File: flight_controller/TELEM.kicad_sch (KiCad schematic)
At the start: 18 parts, among them J13 A1257WV-S-6P-LCP, J14 A1257WV-S-6P-LCP, J15 A1257WV-S-6P-LCP

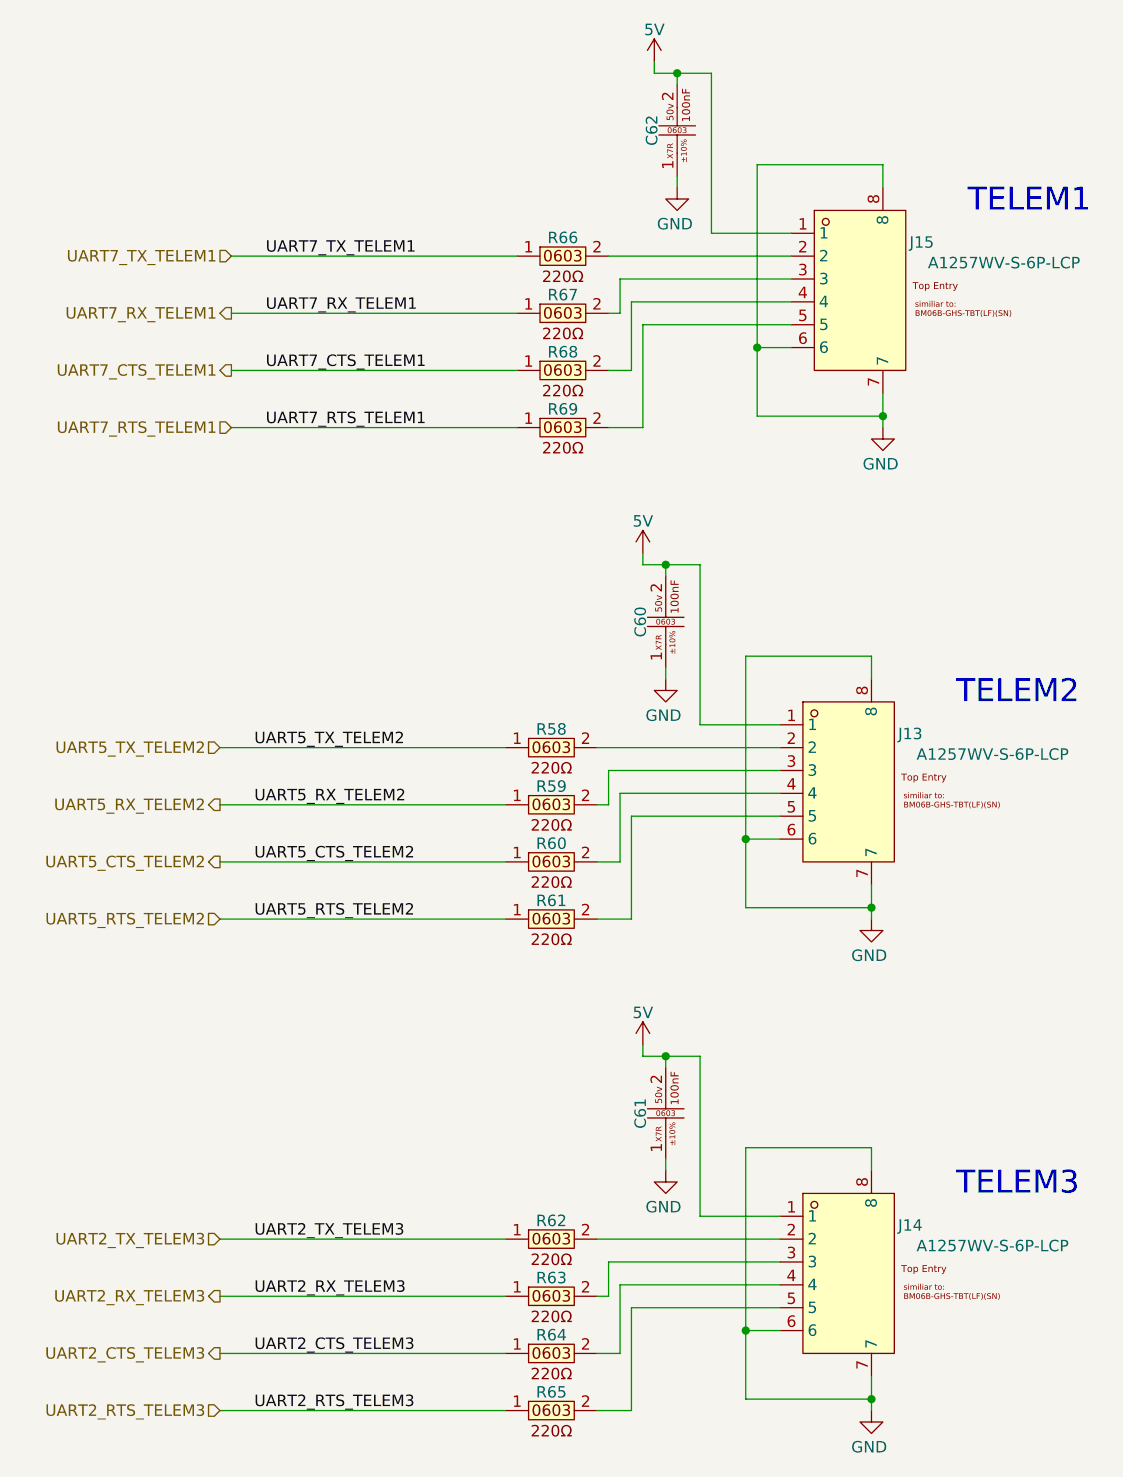
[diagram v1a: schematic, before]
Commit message: Revert to state of commit 2458262 moved all to components to top
Reverts commits: d012532, 3d9c600, 58bc0ac
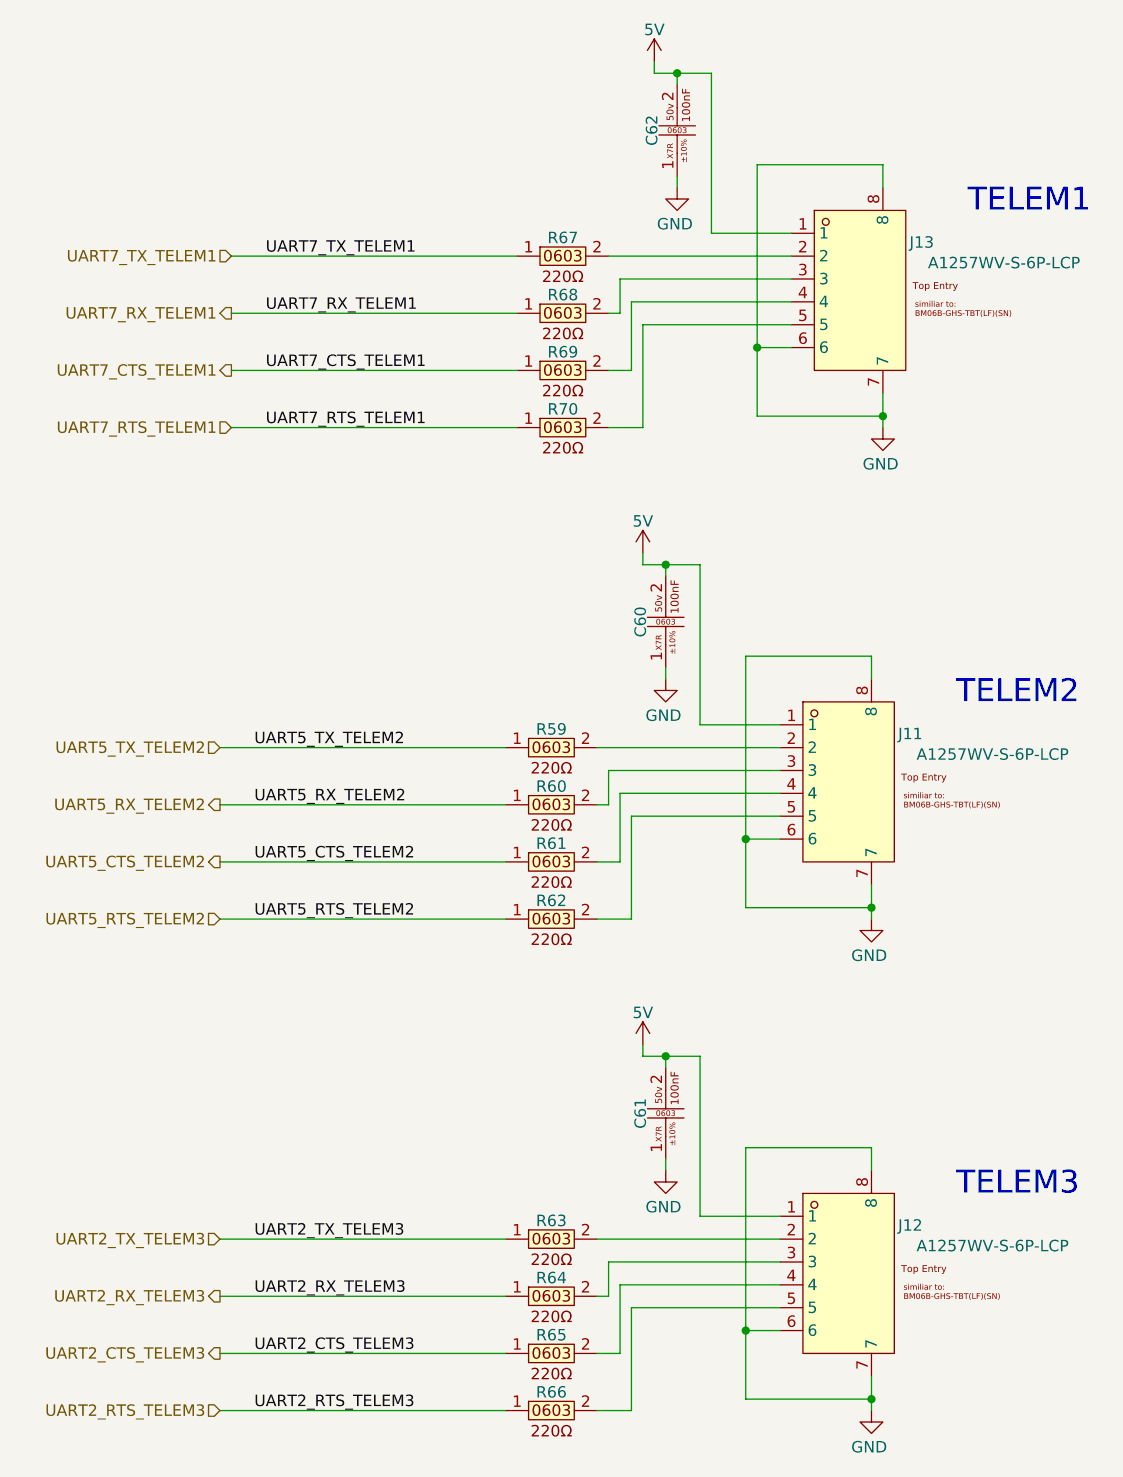
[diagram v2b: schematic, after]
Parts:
- renumbered J13 to J11, J14 to J12, J15 to J13, R58 to R59, R59 to R60, R60 to R61, R61 to R62, R62 to R63, R63 to R64, R64 to R65, R65 to R66, R66 to R67, R67 to R68, R68 to R69, R69 to R70
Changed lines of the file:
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@@
+		(polyline
+			(pts
+				(xy 68.58 129.54) (xy 68.58 181.61) (xy 148.59 181.61) (xy 148.59 129.54)
+			)
+			(stroke
+				(width 0)
+				(type dash)
+			)
+			(fill
+				(type none)
+			)
+		)
+	)
+	(rule_area
 		(polyline
 			(pts
@@
 			(pts
 				(xy 79.375 74.93) (xy 79.375 127) (xy 173.99 127.635) (xy 173.99 74.93)
-			)
-			(stroke
-				(width 0)
-				(type dash)
-			)
-			(fill
-				(type none)
-			)
-		)
-	)
-	(rule_area
-		(polyline
-			(pts
-				(xy 68.58 129.54) (xy 68.58 181.61) (xy 148.59 181.61) (xy 148.59 129.54)
 			)
 			(stroke
@@
 		(dnp no)
 		(fields_autoplaced yes)
-		(property "Reference" "R64"
+		(property "Reference" "R65"
 			(at 85.09 166.878 0)
 			(do_not_autoplace yes)
@@
 			(project "FP_BOARD"
 				(path "/17737359-1a8e-4237-8899-d9604030bc1d/ee742a7d-8184-434b-840f-4020f45cd711"
-					(reference "R64")
+					(reference "R65")
 					(unit 1)
 				)
@@
 		(on_board yes)
 		(dnp no)
-		(property "Reference" "#PWR0158"
+		(property "Reference" "#PWR0160"
 			(at 95.25 138.43 0)
 			(effects
@@
 			(project "FP_BOARD"
 				(path "/17737359-1a8e-4237-8899-d9604030bc1d/ee742a7d-8184-434b-840f-4020f45cd711"
-					(reference "#PWR0158")
+					(reference "#PWR0160")
 					(unit 1)
 				)
@@
 		(dnp no)
 		(fields_autoplaced yes)
-		(property "Reference" "R65"
+		(property "Reference" "R66"
 			(at 85.09 173.228 0)
 			(do_not_autoplace yes)
@@
 			(project "FP_BOARD"
 				(path "/17737359-1a8e-4237-8899-d9604030bc1d/ee742a7d-8184-434b-840f-4020f45cd711"
-					(reference "R65")
+					(reference "R66")
 					(unit 1)
 				)
@@
 		(dnp no)
 		(fields_autoplaced yes)
-		(property "Reference" "R60"
+		(property "Reference" "R61"
 			(at 85.09 112.268 0)
 			(do_not_autoplace yes)
@@
 			(project "FP_BOARD"
 				(path "/17737359-1a8e-4237-8899-d9604030bc1d/ee742a7d-8184-434b-840f-4020f45cd711"
-					(reference "R60")
+					(reference "R61")
 					(unit 1)
 				)
@@
 		(dnp no)
 		(fields_autoplaced yes)
-		(property "Reference" "R62"
+		(property "Reference" "R63"
 			(at 85.09 154.178 0)
 			(do_not_autoplace yes)
@@
 			(project "FP_BOARD"
 				(path "/17737359-1a8e-4237-8899-d9604030bc1d/ee742a7d-8184-434b-840f-4020f45cd711"
-					(reference "R62")
+					(reference "R63")
 					(unit 1)
 				)
@@
 		(dnp no)
 		(fields_autoplaced yes)
-		(property "Reference" "J13"
+		(property "Reference" "J11"
 			(at 124.968 100.076 0)
 			(do_not_autoplace yes)
@@
 			(project "FP_BOARD"
 				(path "/17737359-1a8e-4237-8899-d9604030bc1d/ee742a7d-8184-434b-840f-4020f45cd711"
-					(reference "J13")
+					(reference "J11")
 					(unit 1)
 				)
@@
 		(dnp no)
 		(fields_autoplaced yes)
-		(property "Reference" "J15"
+		(property "Reference" "J13"
 			(at 126.238 45.466 0)
 			(do_not_autoplace yes)
@@
 			(project "FP_BOARD"
 				(path "/17737359-1a8e-4237-8899-d9604030bc1d/ee742a7d-8184-434b-840f-4020f45cd711"
-					(reference "J15")
+					(reference "J13")
 					(unit 1)
 				)
@@
 		(on_board yes)
 		(dnp no)
-		(property "Reference" "#PWR0157"
+		(property "Reference" "#PWR0159"
 			(at 95.25 83.82 0)
 			(effects
@@
 			(project "FP_BOARD"
 				(path "/17737359-1a8e-4237-8899-d9604030bc1d/ee742a7d-8184-434b-840f-4020f45cd711"
-					(reference "#PWR0157")
+					(reference "#PWR0159")
 					(unit 1)
 				)
@@
 		(dnp no)
 		(fields_autoplaced yes)
-		(property "Reference" "J14"
+		(property "Reference" "J12"
 			(at 124.968 154.686 0)
 			(do_not_autoplace yes)
@@
 			(project "FP_BOARD"
 				(path "/17737359-1a8e-4237-8899-d9604030bc1d/ee742a7d-8184-434b-840f-4020f45cd711"
-					(reference "J14")
+					(reference "J12")
 					(unit 1)
 				)
@@
 		(dnp no)
 		(fields_autoplaced yes)
-		(property "Reference" "R63"
+		(property "Reference" "R64"
 			(at 85.09 160.528 0)
 			(do_not_autoplace yes)
@@
 			(project "FP_BOARD"
 				(path "/17737359-1a8e-4237-8899-d9604030bc1d/ee742a7d-8184-434b-840f-4020f45cd711"
-					(reference "R63")
+					(reference "R64")
 					(unit 1)
 				)
@@
 		(dnp no)
 		(fields_autoplaced yes)
-		(property "Reference" "R69"
+		(property "Reference" "R70"
 			(at 86.36 64.008 0)
 			(do_not_autoplace yes)
@@
 			(project "FP_BOARD"
 				(path "/17737359-1a8e-4237-8899-d9604030bc1d/ee742a7d-8184-434b-840f-4020f45cd711"
-					(reference "R69")
+					(reference "R70")
 					(unit 1)
 				)
@@
 		(on_board yes)
 		(dnp no)
-		(property "Reference" "#PWR0161"
+		(property "Reference" "#PWR0163"
 			(at 97.79 154.94 0)
 			(effects
@@
 			(project "FP_BOARD"
 				(path "/17737359-1a8e-4237-8899-d9604030bc1d/ee742a7d-8184-434b-840f-4020f45cd711"
-					(reference "#PWR0161")
+					(reference "#PWR0163")
 					(unit 1)
 				)
@@
 		(dnp no)
 		(fields_autoplaced yes)
-		(property "Reference" "R66"
+		(property "Reference" "R67"
 			(at 86.36 44.958 0)
 			(do_not_autoplace yes)
@@
 			(project "FP_BOARD"
 				(path "/17737359-1a8e-4237-8899-d9604030bc1d/ee742a7d-8184-434b-840f-4020f45cd711"
-					(reference "R66")
+					(reference "R67")
 					(unit 1)
 				)
@@
 		(dnp no)
 		(fields_autoplaced yes)
-		(property "Reference" "R61"
+		(property "Reference" "R62"
 			(at 85.09 118.618 0)
 			(do_not_autoplace yes)
@@
 			(project "FP_BOARD"
 				(path "/17737359-1a8e-4237-8899-d9604030bc1d/ee742a7d-8184-434b-840f-4020f45cd711"
-					(reference "R61")
+					(reference "R62")
 					(unit 1)
 				)
@@
 		(dnp no)
 		(fields_autoplaced yes)
-		(property "Reference" "R58"
+		(property "Reference" "R59"
 			(at 85.09 99.568 0)
 			(do_not_autoplace yes)
@@
 			(project "FP_BOARD"
 				(path "/17737359-1a8e-4237-8899-d9604030bc1d/ee742a7d-8184-434b-840f-4020f45cd711"
-					(reference "R58")
+					(reference "R59")
 					(unit 1)
 				)
@@
 		(on_board yes)
 		(dnp no)
-		(property "Reference" "#PWR0164"
+		(property "Reference" "#PWR0166"
 			(at 120.65 181.61 0)
 			(effects
@@
 			(project "FP_BOARD"
 				(path "/17737359-1a8e-4237-8899-d9604030bc1d/ee742a7d-8184-434b-840f-4020f45cd711"
-					(reference "#PWR0164")
+					(reference "#PWR0166")
 					(unit 1)
 				)
@@
 		(on_board yes)
 		(dnp no)
-		(property "Reference" "#PWR0160"
+		(property "Reference" "#PWR0162"
 			(at 97.79 100.33 0)
 			(effects
@@
 			(project "FP_BOARD"
 				(path "/17737359-1a8e-4237-8899-d9604030bc1d/ee742a7d-8184-434b-840f-4020f45cd711"
-					(reference "#PWR0160")
+					(reference "#PWR0162")
 					(unit 1)
 				)
@@
 		(dnp no)
 		(fields_autoplaced yes)
-		(property "Reference" "R67"
+		(property "Reference" "R68"
 			(at 86.36 51.308 0)
 			(do_not_autoplace yes)
@@
 			(project "FP_BOARD"
 				(path "/17737359-1a8e-4237-8899-d9604030bc1d/ee742a7d-8184-434b-840f-4020f45cd711"
-					(reference "R67")
+					(reference "R68")
 					(unit 1)
 				)
@@
 		(dnp no)
 		(fields_autoplaced yes)
-		(property "Reference" "R68"
+		(property "Reference" "R69"
 			(at 86.36 57.658 0)
 			(do_not_autoplace yes)
@@
 			(project "FP_BOARD"
 				(path "/17737359-1a8e-4237-8899-d9604030bc1d/ee742a7d-8184-434b-840f-4020f45cd711"
-					(reference "R68")
+					(reference "R69")
 					(unit 1)
 				)
@@
 		(on_board yes)
 		(dnp no)
-		(property "Reference" "#PWR0163"
+		(property "Reference" "#PWR0165"
 			(at 120.65 127 0)
 			(effects
@@
 			(project "FP_BOARD"
 				(path "/17737359-1a8e-4237-8899-d9604030bc1d/ee742a7d-8184-434b-840f-4020f45cd711"
-					(reference "#PWR0163")
+					(reference "#PWR0165")
 					(unit 1)
 				)
@@
 		(dnp no)
 		(fields_autoplaced yes)
-		(property "Reference" "R59"
+		(property "Reference" "R60"
 			(at 85.09 105.918 0)
 			(do_not_autoplace yes)
@@
 			(project "FP_BOARD"
 				(path "/17737359-1a8e-4237-8899-d9604030bc1d/ee742a7d-8184-434b-840f-4020f45cd711"
-					(reference "R59")
+					(reference "R60")
 					(unit 1)
 				)
@@
 		(on_board yes)
 		(dnp no)
-		(property "Reference" "#PWR0162"
+		(property "Reference" "#PWR0164"
 			(at 99.06 45.72 0)
 			(effects
@@
 			(project "FP_BOARD"
 				(path "/17737359-1a8e-4237-8899-d9604030bc1d/ee742a7d-8184-434b-840f-4020f45cd711"
-					(reference "#PWR0162")
+					(reference "#PWR0164")
 					(unit 1)
 				)
@@
 		(on_board yes)
 		(dnp no)
-		(property "Reference" "#PWR0159"
+		(property "Reference" "#PWR0161"
 			(at 96.52 29.21 0)
 			(effects
@@
 			(project "FP_BOARD"
 				(path "/17737359-1a8e-4237-8899-d9604030bc1d/ee742a7d-8184-434b-840f-4020f45cd711"
-					(reference "#PWR0159")
+					(reference "#PWR0161")
 					(unit 1)
 				)
@@
 		(on_board yes)
 		(dnp no)
-		(property "Reference" "#PWR0165"
+		(property "Reference" "#PWR0167"
 			(at 121.92 72.39 0)
 			(effects
@@
 			(project "FP_BOARD"
 				(path "/17737359-1a8e-4237-8899-d9604030bc1d/ee742a7d-8184-434b-840f-4020f45cd711"
-					(reference "#PWR0165")
-					(unit 1)
-				)
+					(reference "#PWR0167")
+					(unit 1)
+				)
